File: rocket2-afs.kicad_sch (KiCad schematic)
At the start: 68 parts, among them J1 ARMING_PLUG, J2 POWER, J3 E-MATCH_DROGUE, J4 SWD, J5 E-MATCH_RECOVERY, Q1 Q_NMOS_GSD, Q2 Q_NMOS_GSD, Q3 Q_NMOS_GSD, Q4 Q_NMOS_GSD, Q5 Q_NMOS_GSD, U2 LD1086DT33TR, U8 USBLC6-2SC6, Y1 16MHz

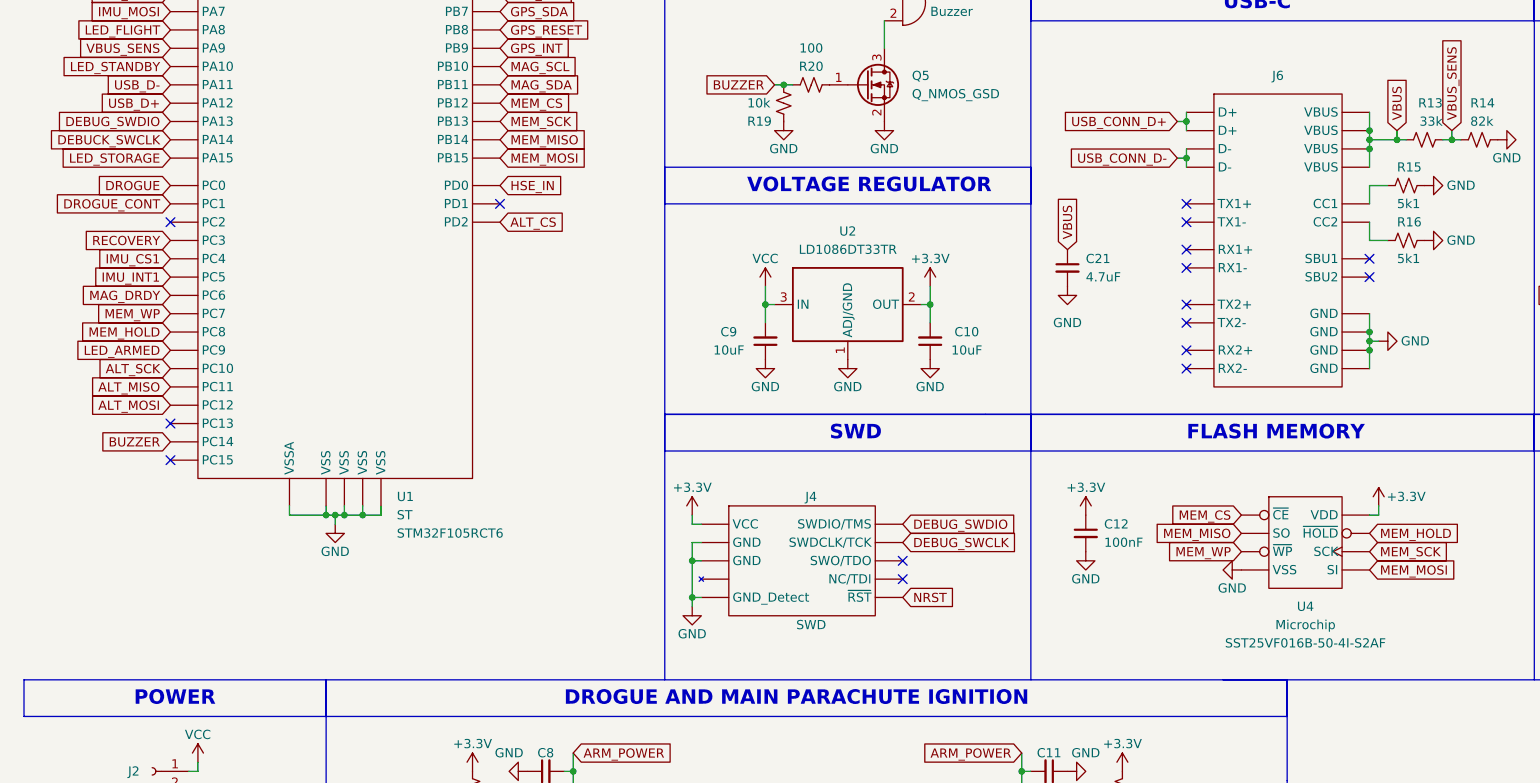
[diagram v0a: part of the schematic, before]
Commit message: Final tweaks
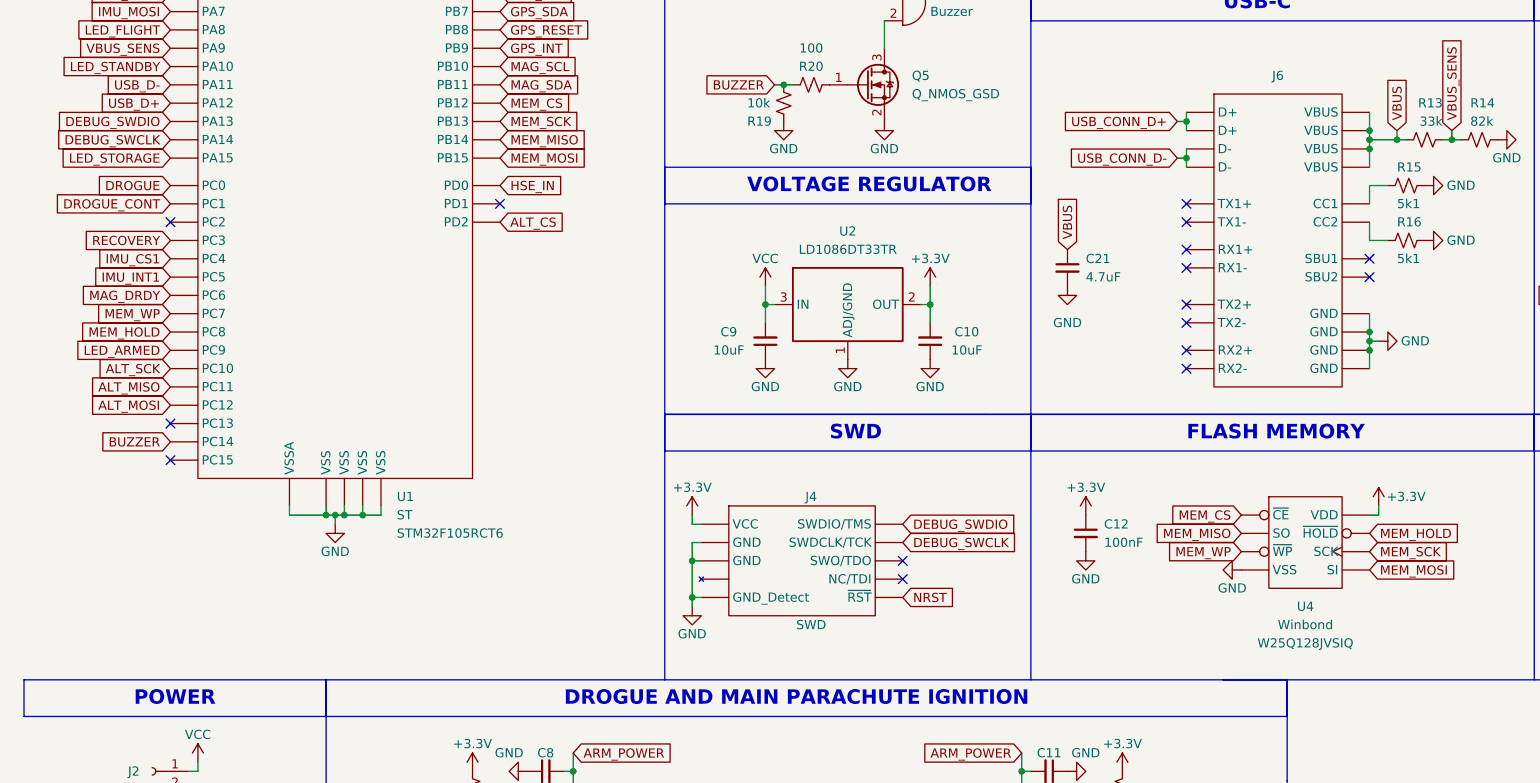
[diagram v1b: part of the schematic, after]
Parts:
- C1, C11, C12, C13, C14, C15, C16, C17, C18, C19, C2, C20, C3, C4, C5, C6, C7, C8: Part # Generic 0603 6.3V 100nF X7R MLCC Capacitor -> Generic 0603 6.3V 100nF X7R MLCC
- C10, C9: Part # Generic 0603 6.3V 10uF X7R MLCC Capacitor -> Generic 0603 6.3V 10uF X7R MLCC
- C21: Part # Generic 0603 6.3V 4.7nF X7R MLCC Capacitor -> Generic 0603 6.3V 4.7uF X7R MLCC
- J4: Part # Generic 2x05 P1.27mm Vertical SMD -> Generic 2x05 P1.27mm Vertical Pin Header SMD
- U4: Manufacturer Microchip -> Winbond; Part # SST25VF016B-50-4I-S2AF -> W25Q128JVSIQ
- Y1: Manufacturer RoHS -> ECS; Part # ECS-1633 -> ECS-1633-160-BN-TR
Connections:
- net DEBUCK_SWCLK is gone; now on net DEBUG_SWCLK: U1.49 (PA14)
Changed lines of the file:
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@@
     )
   )
-  (global_label "DEBUCK_SWCLK" (shape input) (at 33.02 92.71 180) (fields_autoplaced)
+  (global_label "DEBUG_SWCLK" (shape input) (at 33.02 92.71 180) (fields_autoplaced)
     (effects (font (size 1.27 1.27)) (justify right))
-    (property "Intersheetrefs" "${INTERSHEET_REFS}" (at 15.2787 92.71 0)
+    (property "Intersheetrefs" "${INTERSHEET_REFS}" (at 16.5487 92.71 0)
       (effects (font (size 1.27 1.27)) (justify right) hide)
     )
@@
       (effects (font (size 1.27 1.27)) hide)
     )
-    (property "Part #" "Generic 0603 6.3V 100nF X7R MLCC Capacitor" (at 274.32 90.17 0)
+    (property "Part #" "Generic 0603 6.3V 100nF X7R MLCC" (at 274.32 90.17 0)
       (effects (font (size 1.27 1.27)) hide)
     )
@@
       (effects (font (size 1.27 1.27)) hide)
     )
-    (property "Part #" "Generic 0603 6.3V 100nF X7R MLCC Capacitor" (at 38.1 26.67 0)
+    (property "Part #" "Generic 0603 6.3V 100nF X7R MLCC" (at 38.1 26.67 0)
       (effects (font (size 1.27 1.27)) hide)
     )
@@
       (effects (font (size 1.27 1.27)) hide)
     )
-    (property "Part #" "Generic 0603 6.3V 100nF X7R MLCC Capacitor" (at 154.94 180.34 0)
+    (property "Part #" "Generic 0603 6.3V 100nF X7R MLCC" (at 154.94 180.34 0)
       (effects (font (size 1.27 1.27)) hide)
     )
@@
       (effects (font (size 1.27 1.27)) hide)
     )
-    (property "Part #" "Generic 0603 6.3V 10uF X7R MLCC Capacitor" (at 138.43 120.65 0)
+    (property "Part #" "Generic 0603 6.3V 10uF X7R MLCC" (at 138.43 120.65 0)
       (effects (font (size 1.27 1.27)) hide)
     )
@@
       (effects (font (size 1.27 1.27)) hide)
     )
-    (property "Part #" "Generic 0603 6.3V 100nF X7R MLCC Capacitor" (at 72.39 26.67 0)
+    (property "Part #" "Generic 0603 6.3V 100nF X7R MLCC" (at 72.39 26.67 0)
       (effects (font (size 1.27 1.27)) hide)
     )
@@
       (effects (font (size 1.27 1.27)) hide)
     )
-    (property "Part #" "Generic 0603 6.3V 100nF X7R MLCC Capacitor" (at 160.02 147.32 0)
+    (property "Part #" "Generic 0603 6.3V 100nF X7R MLCC" (at 160.02 147.32 0)
       (effects (font (size 1.27 1.27)) hide)
     )
@@
       (effects (font (size 1.27 1.27)) hide)
     )
-    (property "Part #" "Generic 0603 6.3V 100nF X7R MLCC Capacitor" (at 85.09 180.34 0)
+    (property "Part #" "Generic 0603 6.3V 100nF X7R MLCC" (at 85.09 180.34 0)
       (effects (font (size 1.27 1.27)) hide)
     )
@@
       (effects (font (size 1.27 1.27)) hide)
     )
-    (property "Manufacturer" "RoHS" (at 87.63 45.72 0)
+    (property "Manufacturer" "ECS" (at 87.63 45.72 0)
       (effects (font (size 1.27 1.27)) hide)
     )
-    (property "Part #" "ECS-1633" (at 87.63 45.72 0)
+    (property "Part #" "ECS-1633-160-BN-TR" (at 87.63 45.72 0)
       (effects (font (size 1.27 1.27)) hide)
     )
@@
       (effects (font (size 1.27 1.27)) hide)
     )
-    (property "Part #" "Generic 2x05 P1.27mm Vertical SMD" (at 120.65 151.13 0)
+    (property "Part #" "Generic 2x05 P1.27mm Vertical Pin Header SMD" (at 120.65 151.13 0)
       (effects (font (size 1.27 1.27)) hide)
     )
@@
       (effects (font (size 1.27 1.27)) hide)
     )
-    (property "Part #" "Generic 0603 6.3V 100nF X7R MLCC Capacitor" (at 83.82 26.67 0)
+    (property "Part #" "Generic 0603 6.3V 100nF X7R MLCC" (at 83.82 26.67 0)
       (effects (font (size 1.27 1.27)) hide)
     )
@@
       (effects (font (size 1.27 1.27)) hide)
     )
-    (property "Part #" "Generic 0603 6.3V 100nF X7R MLCC Capacitor" (at 213.36 26.67 0)
+    (property "Part #" "Generic 0603 6.3V 100nF X7R MLCC" (at 213.36 26.67 0)
       (effects (font (size 1.27 1.27)) hide)
     )
@@
       (effects (font (size 1.27 1.27)) hide)
     )
-    (property "Part #" "Generic 0603 6.3V 100nF X7R MLCC Capacitor" (at 60.96 26.67 0)
+    (property "Part #" "Generic 0603 6.3V 100nF X7R MLCC" (at 60.96 26.67 0)
       (effects (font (size 1.27 1.27)) hide)
     )
@@
       (effects (font (size 1.27 1.27)) hide)
     )
-    (property "Part #" "Generic 0603 6.3V 100nF X7R MLCC Capacitor" (at 49.53 26.67 0)
+    (property "Part #" "Generic 0603 6.3V 100nF X7R MLCC" (at 49.53 26.67 0)
       (effects (font (size 1.27 1.27)) hide)
     )
@@
       (effects (font (size 1.27 1.27)) hide)
     )
-    (property "Part #" "Generic 0603 6.3V 100nF X7R MLCC Capacitor" (at 21.59 52.07 0)
+    (property "Part #" "Generic 0603 6.3V 100nF X7R MLCC" (at 21.59 52.07 0)
       (effects (font (size 1.27 1.27)) hide)
     )
@@
       (effects (font (size 1.27 1.27)) hide)
     )
-    (property "Part #" "Generic 0603 6.3V 100nF X7R MLCC Capacitor" (at 252.73 90.17 0)
+    (property "Part #" "Generic 0603 6.3V 100nF X7R MLCC" (at 252.73 90.17 0)
       (effects (font (size 1.27 1.27)) hide)
     )
@@
       (effects (font (size 1.27 1.27)) hide)
     )
-    (property "Part #" "Generic 0603 6.3V 10uF X7R MLCC Capacitor" (at 115.57 120.65 0)
+    (property "Part #" "Generic 0603 6.3V 10uF X7R MLCC" (at 115.57 120.65 0)
       (effects (font (size 1.27 1.27)) hide)
     )
@@
       (effects (font (size 1.27 1.27)) hide)
     )
-    (property "Part #" "Generic 0603 6.3V 100nF X7R MLCC Capacitor" (at 238.76 27.94 0)
+    (property "Part #" "Generic 0603 6.3V 100nF X7R MLCC" (at 238.76 27.94 0)
       (effects (font (size 1.27 1.27)) hide)
     )
@@
       (effects (font (size 1.27 1.27)) hide)
     )
-    (property "Part #" "Generic 0603 6.3V 4.7nF X7R MLCC Capacitor" (at 157.48 110.49 0)
+    (property "Part #" "Generic 0603 6.3V 4.7uF X7R MLCC" (at 157.48 110.49 0)
       (effects (font (size 1.27 1.27)) hide)
     )
@@
       (effects (font (size 1.27 1.27)) hide)
     )
-    (property "Part #" "Generic 0603 6.3V 100nF X7R MLCC Capacitor" (at 190.5 26.67 0)
+    (property "Part #" "Generic 0603 6.3V 100nF X7R MLCC" (at 190.5 26.67 0)
       (effects (font (size 1.27 1.27)) hide)
     )
@@
       (effects (font (size 1.27 1.27)) hide)
     )
-    (property "Datasheet" "https://ww1.microchip.com/downloads/en/DeviceDoc/20005044C.pdf" (at 190.5 148.59 0)
+    (property "Datasheet" "https://www.winbond.com/resource-files/W25Q128JV%20RevI%2008232021%20Plus.pdf" (at 190.5 148.59 0)
       (effects (font (size 1.27 1.27)) hide)
     )
-    (property "Manufacturer" "Microchip" (at 190.5 160.02 0)
+    (property "Manufacturer" "Winbond" (at 190.5 160.02 0)
       (effects (font (size 1.27 1.27)))
     )
-    (property "Part #" "SST25VF016B-50-4I-S2AF" (at 190.5 162.56 0)
+    (property "Part #" "W25Q128JVSIQ" (at 190.5 162.56 0)
       (effects (font (size 1.27 1.27)))
     )
@@
       (effects (font (size 1.27 1.27)) hide)
     )
-    (property "Part #" "Generic 0603 6.3V 100nF X7R MLCC Capacitor" (at 228.6 146.05 0)
+    (property "Part #" "Generic 0603 6.3V 100nF X7R MLCC" (at 228.6 146.05 0)
       (effects (font (size 1.27 1.27)) hide)
     )
@@
       (effects (font (size 1.27 1.27)) hide)
     )
-    (property "Datasheet" "https://www.we-online.com/components/products/datasheet/629105150521.pdf" (at 186.69 106.68 0)
+    (property "Datasheet" "https://gct.co/files/drawings/usb4105.pdf?v=5f9eb85e-7d29-4c03-ba83-51194e8d0df3" (at 186.69 106.68 0)
       (effects (font (size 1.27 1.27)) hide)
     )
@@
       (effects (font (size 1.27 1.27)) hide)
     )
-    (property "Part #" "Generic 0603 6.3V 100nF X7R MLCC Capacitor" (at 227.33 27.94 0)
+    (property "Part #" "Generic 0603 6.3V 100nF X7R MLCC" (at 227.33 27.94 0)
       (effects (font (size 1.27 1.27)) hide)
     )
@@
       (effects (font (size 1.27 1.27)) hide)
     )
-    (property "Part #" "Generic 0603 6.3V 100nF X7R MLCC Capacitor" (at 201.93 26.67 0)
+    (property "Part #" "Generic 0603 6.3V 100nF X7R MLCC" (at 201.93 26.67 0)
       (effects (font (size 1.27 1.27)) hide)
     )
@@
       (effects (font (size 1.27 1.27)) hide)
     )
-    (property "Part #" "Generic 0603 6.3V 100nF X7R MLCC Capacitor" (at 26.67 26.67 0)
+    (property "Part #" "Generic 0603 6.3V 100nF X7R MLCC" (at 26.67 26.67 0)
       (effects (font (size 1.27 1.27)) hide)
     )
